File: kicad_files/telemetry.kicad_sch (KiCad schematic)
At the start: 24 parts, among them J3 RFD900ux 10 Pin Header, J4 Conn_ARM_JTAG_SWD_10, J5 RFD900ux 3 Pin Power Select, J6 USB_C_Receptacle_USB2.0_16P, U8 74AHCT125, U9 WE-TVS-82400102

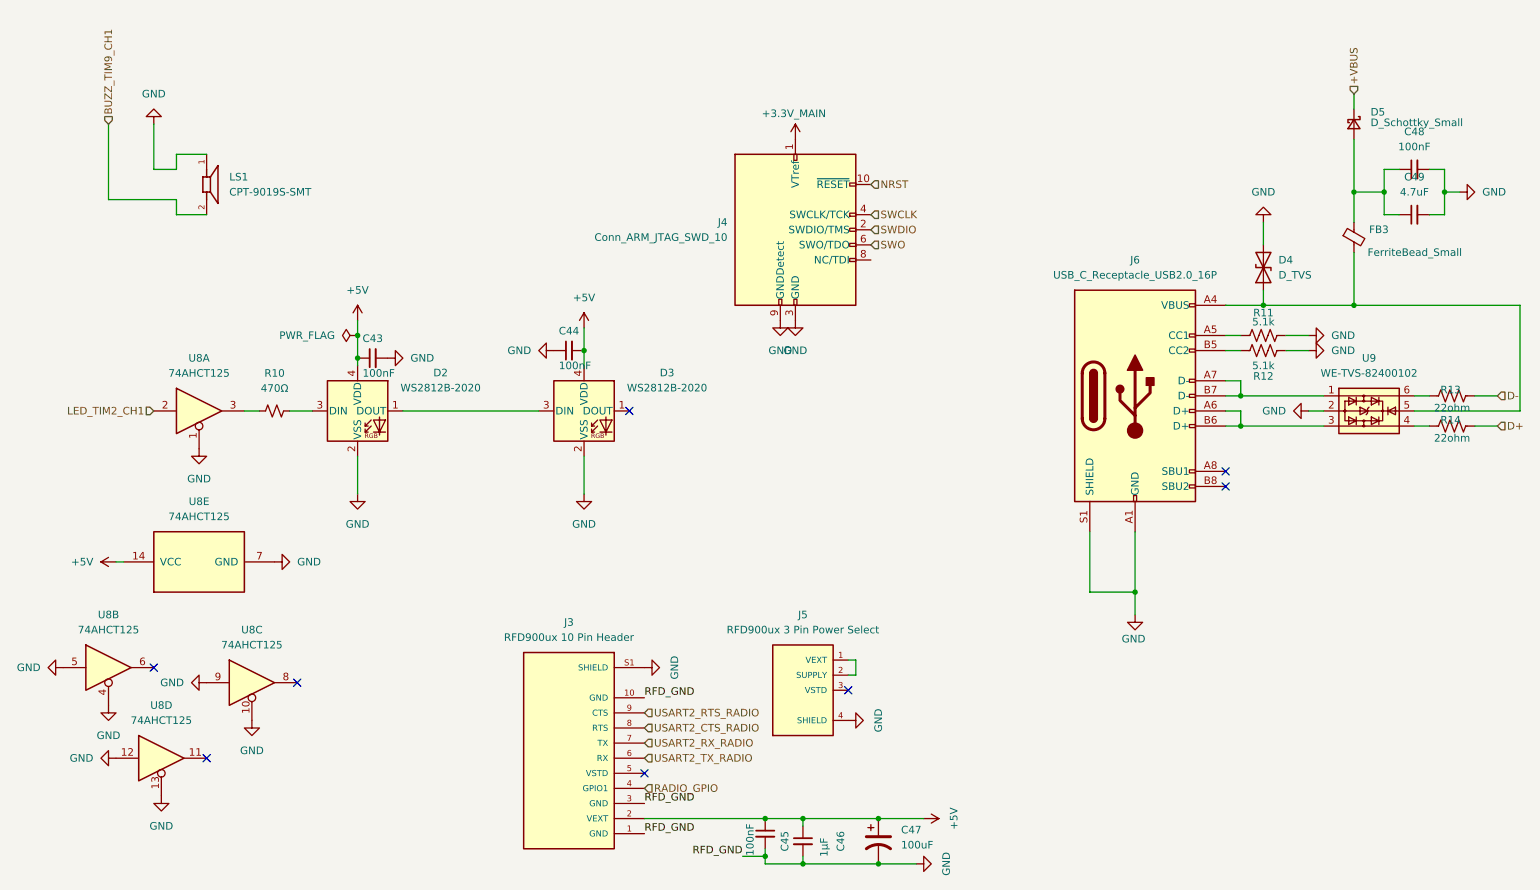
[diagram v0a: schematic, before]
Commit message: make schematic changes
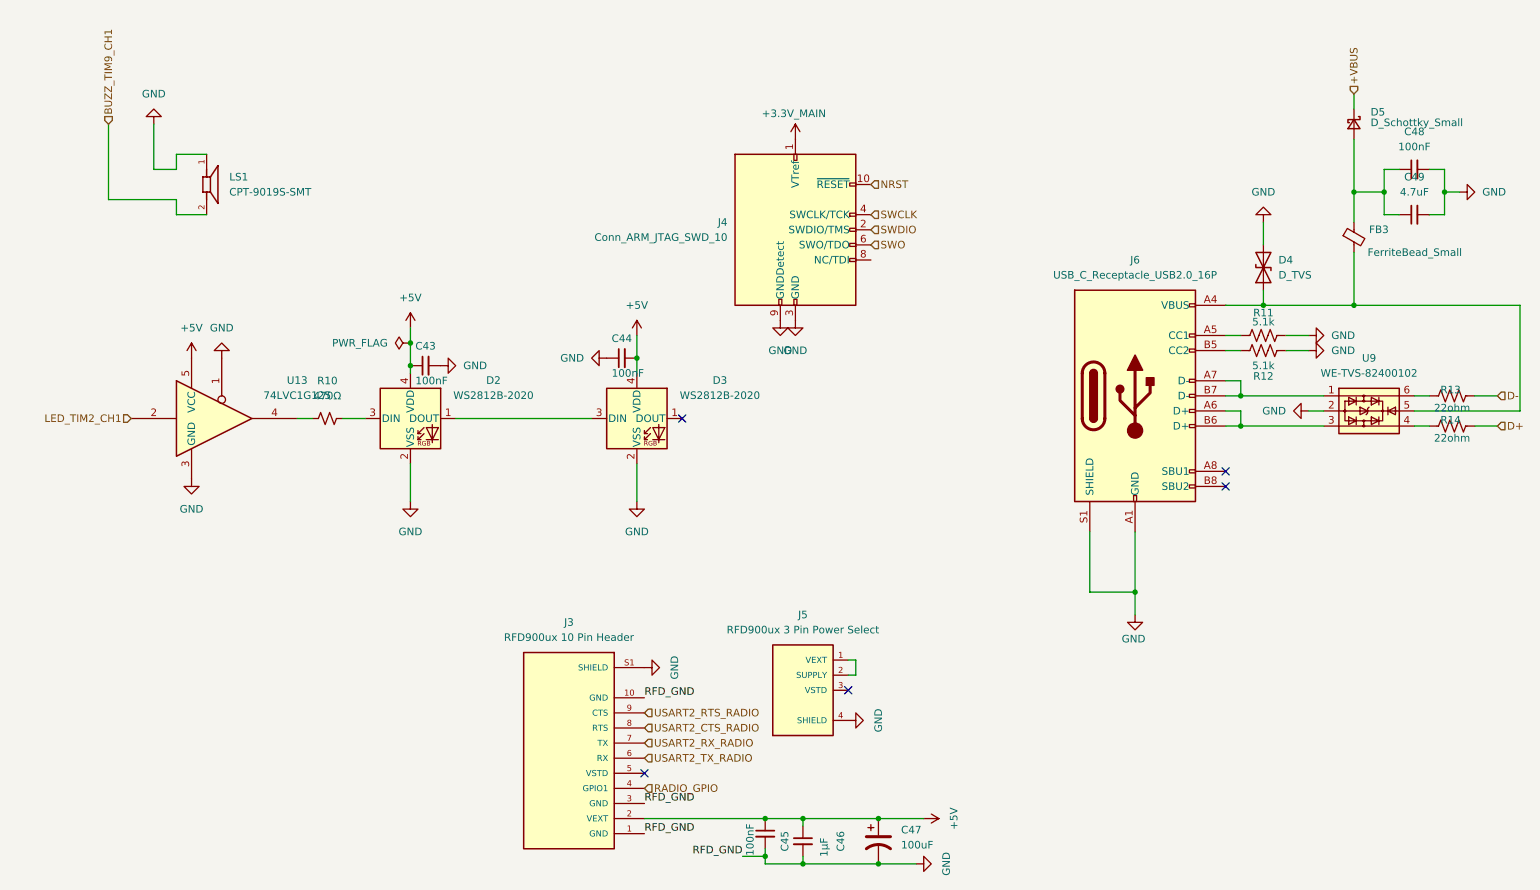
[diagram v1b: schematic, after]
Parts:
- removed U8: 74AHCT125, Package_SO:SOIC-14_3.9x8.7mm_P1.27mm, symbol 74xx:74AHCT125
- added U13: 74LVC1G125, Package_TO_SOT_SMD:SOT-23-5, symbol 74xGxx:74LVC1G125
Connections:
- net +5V: now also U13.5 (VCC)
- net GND: now also U13.1, U13.3 (GND)
- net LED_TIM2_CH1: now also U13.2
- net at R10.1: now also U13.4
- no-connect marks 8 -> 5
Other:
- moved on the sheet: C43, C44, D2, D3, R10
